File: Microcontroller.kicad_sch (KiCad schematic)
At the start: 87 parts, among them J2 2.54 mm header, J3 Conn_01x14_Pin, J4 HX JN1.27-2x5 WZ H4.9, J5 USB_C_Receptacle_USB2.0_16P, U2 STM32G431K8Tx, U4 USBLC6-2SC6, Y1 20 MHz

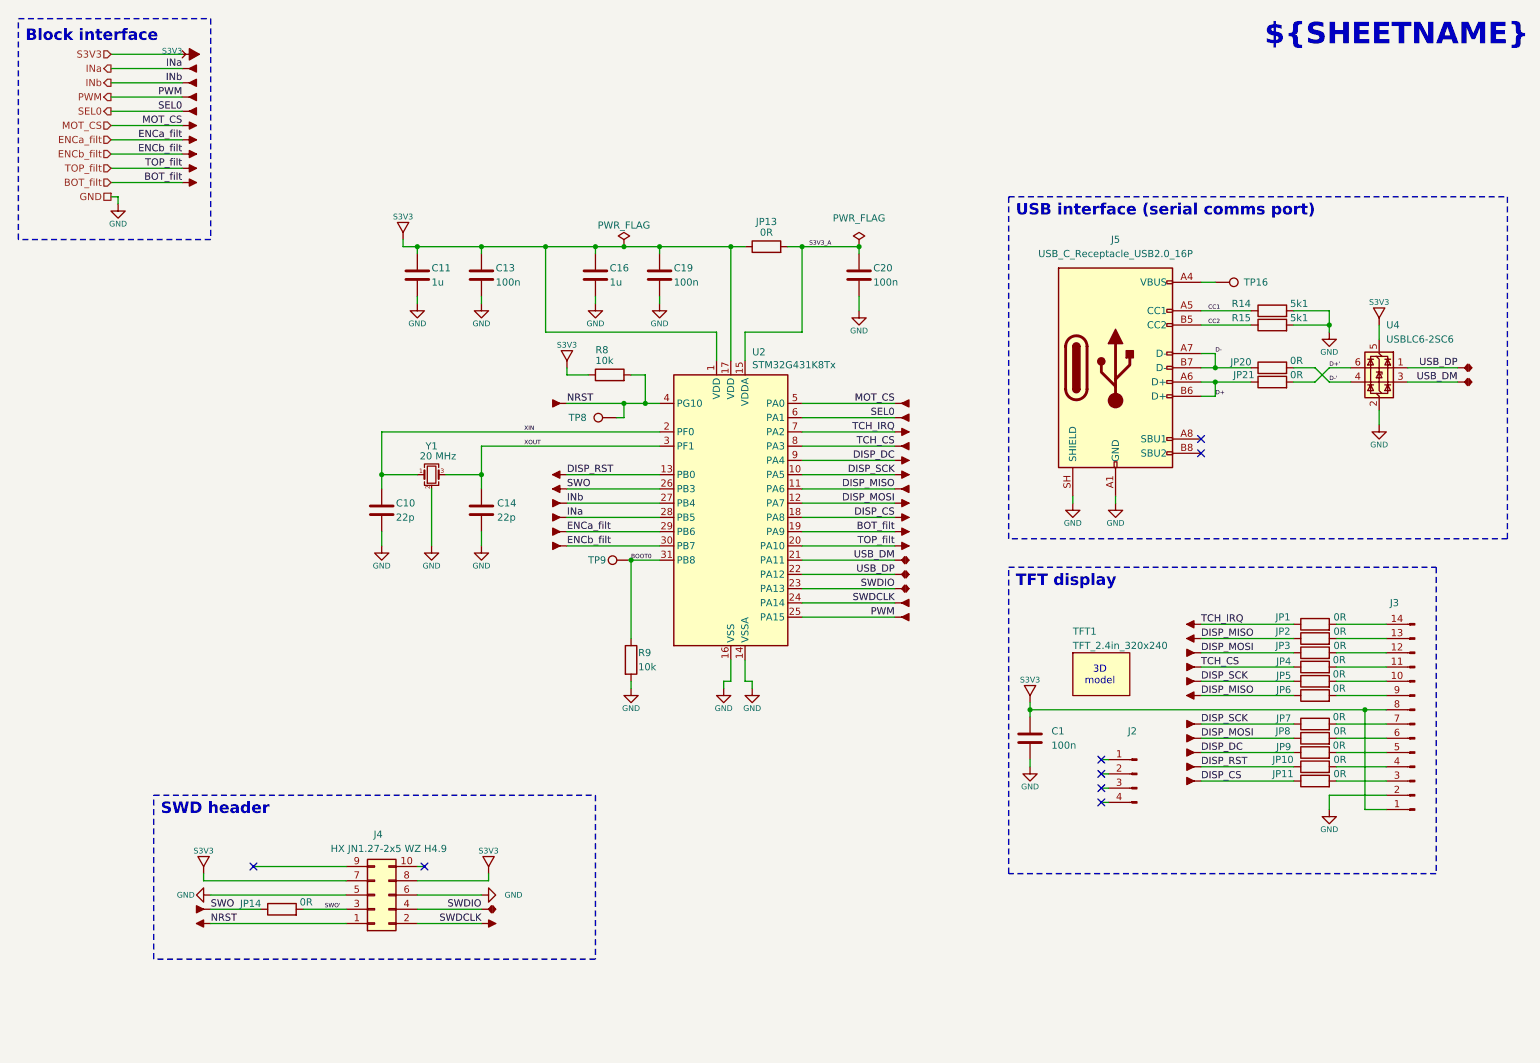
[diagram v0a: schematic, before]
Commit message: sch update
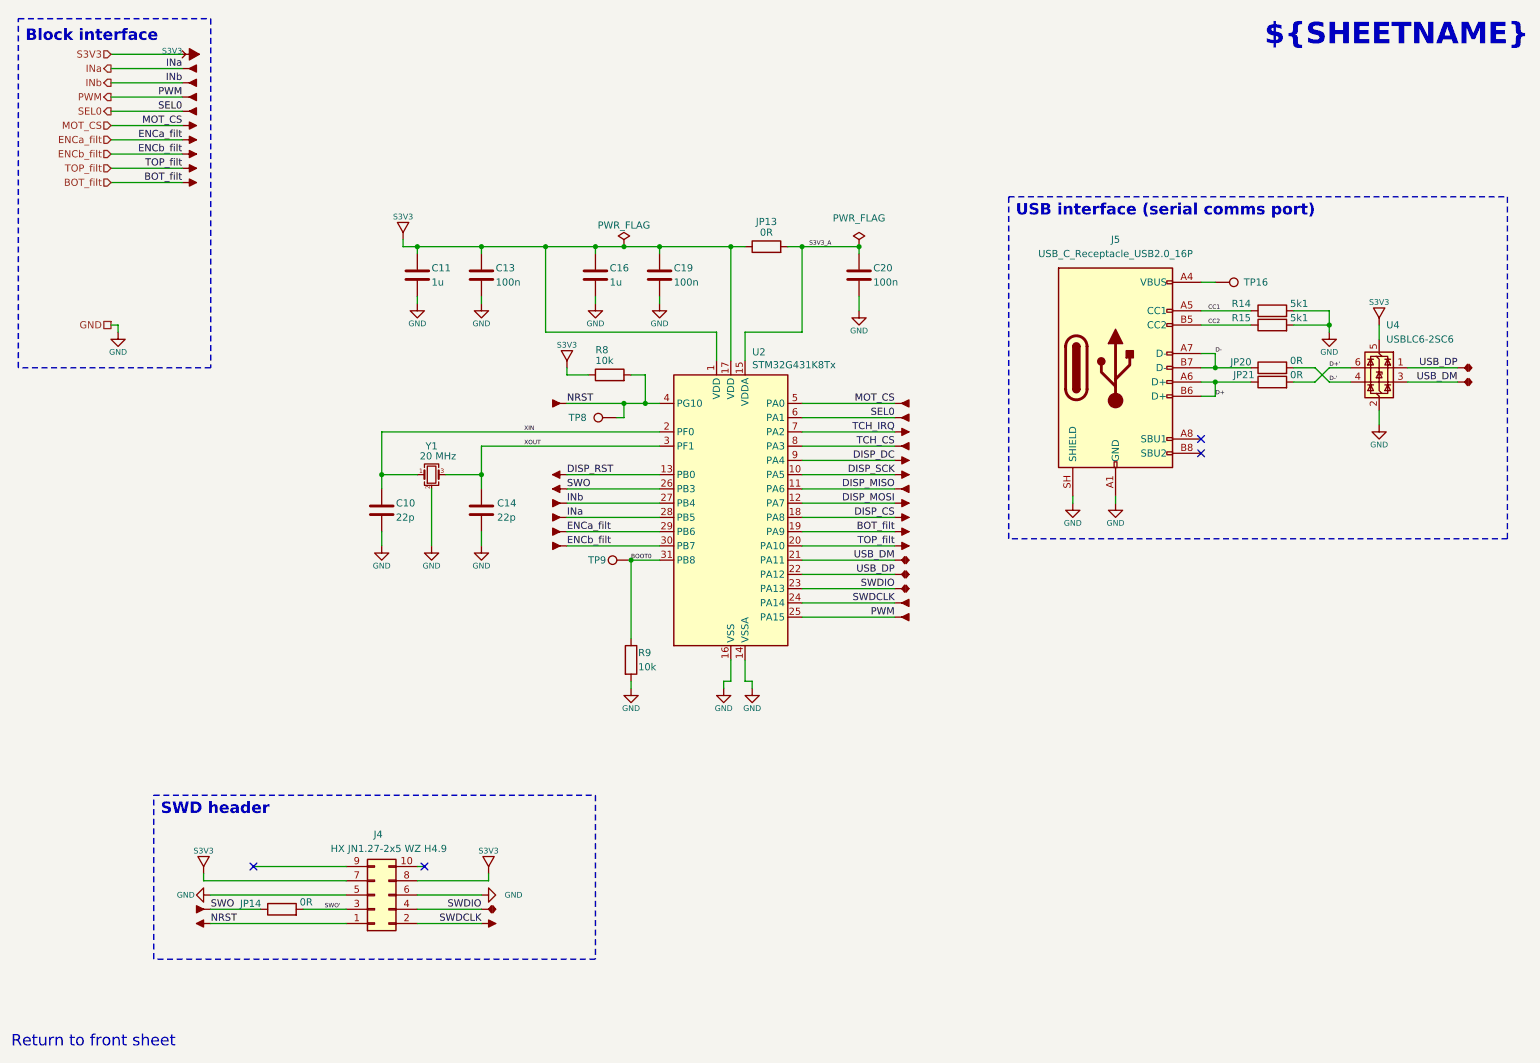
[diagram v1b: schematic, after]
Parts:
- removed C1: 100n, Capacitor_SMD:C_0603_1608Metric_Pad1.08x0.95mm_HandSolder, symbol Device:C
- removed J2: 2.54 mm header, Connector_PinSocket_2.54mm:PinSocket_1x04_P2.54mm_Vertical, symbol Connector:Conn_01x04_Pin
- removed J3: Conn_01x14_Pin, Connector_PinSocket_2.54mm:PinSocket_1x14_P2.54mm_Vertical, symbol Connector:Conn_01x14_Pin
- removed JP1, JP10, JP11, JP2, JP3, JP8: 0R, Personal:Jumper_0603, symbol Device:R
- removed JP4, JP5, JP7: 0R, Resistor_SMD:R_1206_3216Metric_Pad1.30x1.75mm_HandSolder, symbol Device:R
- removed JP6: 0R, Resistor_SMD:R_0603_1608Metric_Pad0.98x0.95mm_HandSolder, symbol Device:R
- removed JP9: 0R, Resistor_THT:R_Axial_DIN0204_L3.6mm_D1.6mm_P5.08mm_Horizontal, symbol Device:R
- removed P1, P2, P6: (no value), symbol personal:Cosmetic_OUT
- removed P10, P11, P3, P4, P5, P7, P8, P9: (no value), symbol personal:Cosmetic_IN
- removed TFT1: TFT_2.4in_320x240, Personal:Display_240x320_ILI9341_2.4in_no_pads, symbol personal:TFT_2.8_IN_320x240
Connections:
- no-connect marks 8 -> 4
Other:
- note added: "Return to front sheet"
- note removed: "3D model"
- note removed: "TFT display"

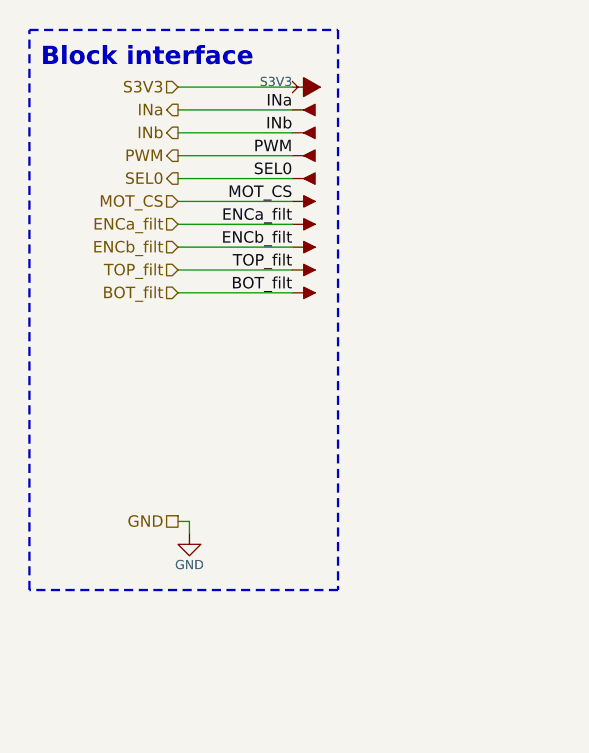
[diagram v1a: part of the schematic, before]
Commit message: sch2
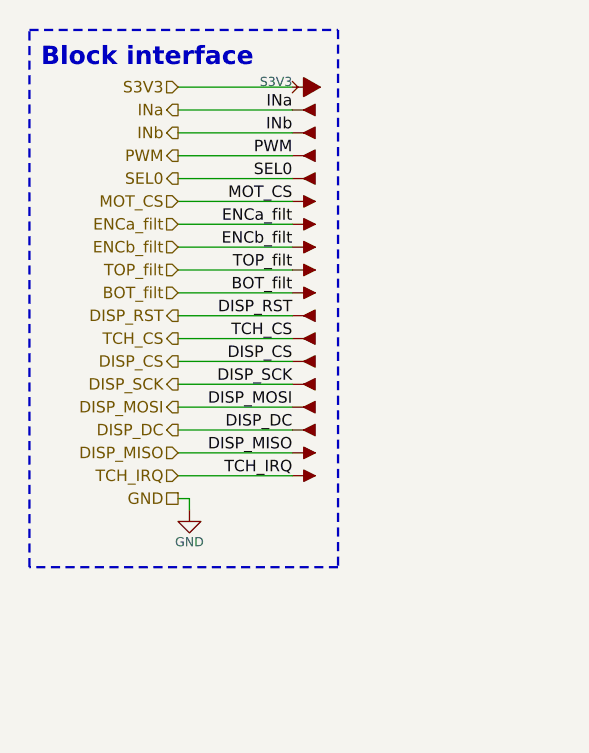
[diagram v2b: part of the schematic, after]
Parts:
- added P100, P101: (no value), symbol personal:Cosmetic_OUT
- added P94, P95, P96, P97, P98, P99: (no value), symbol personal:Cosmetic_IN
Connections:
- net DISP_CS: now also P96.1
- net DISP_DC: now also P99.1
- net DISP_MISO: now also P100.1
- net DISP_MOSI: now also P98.1
- net DISP_RST: now also P94.1
- net DISP_SCK: now also P97.1
- net TCH_CS: now also P95.1
- net TCH_IRQ: now also P101.1

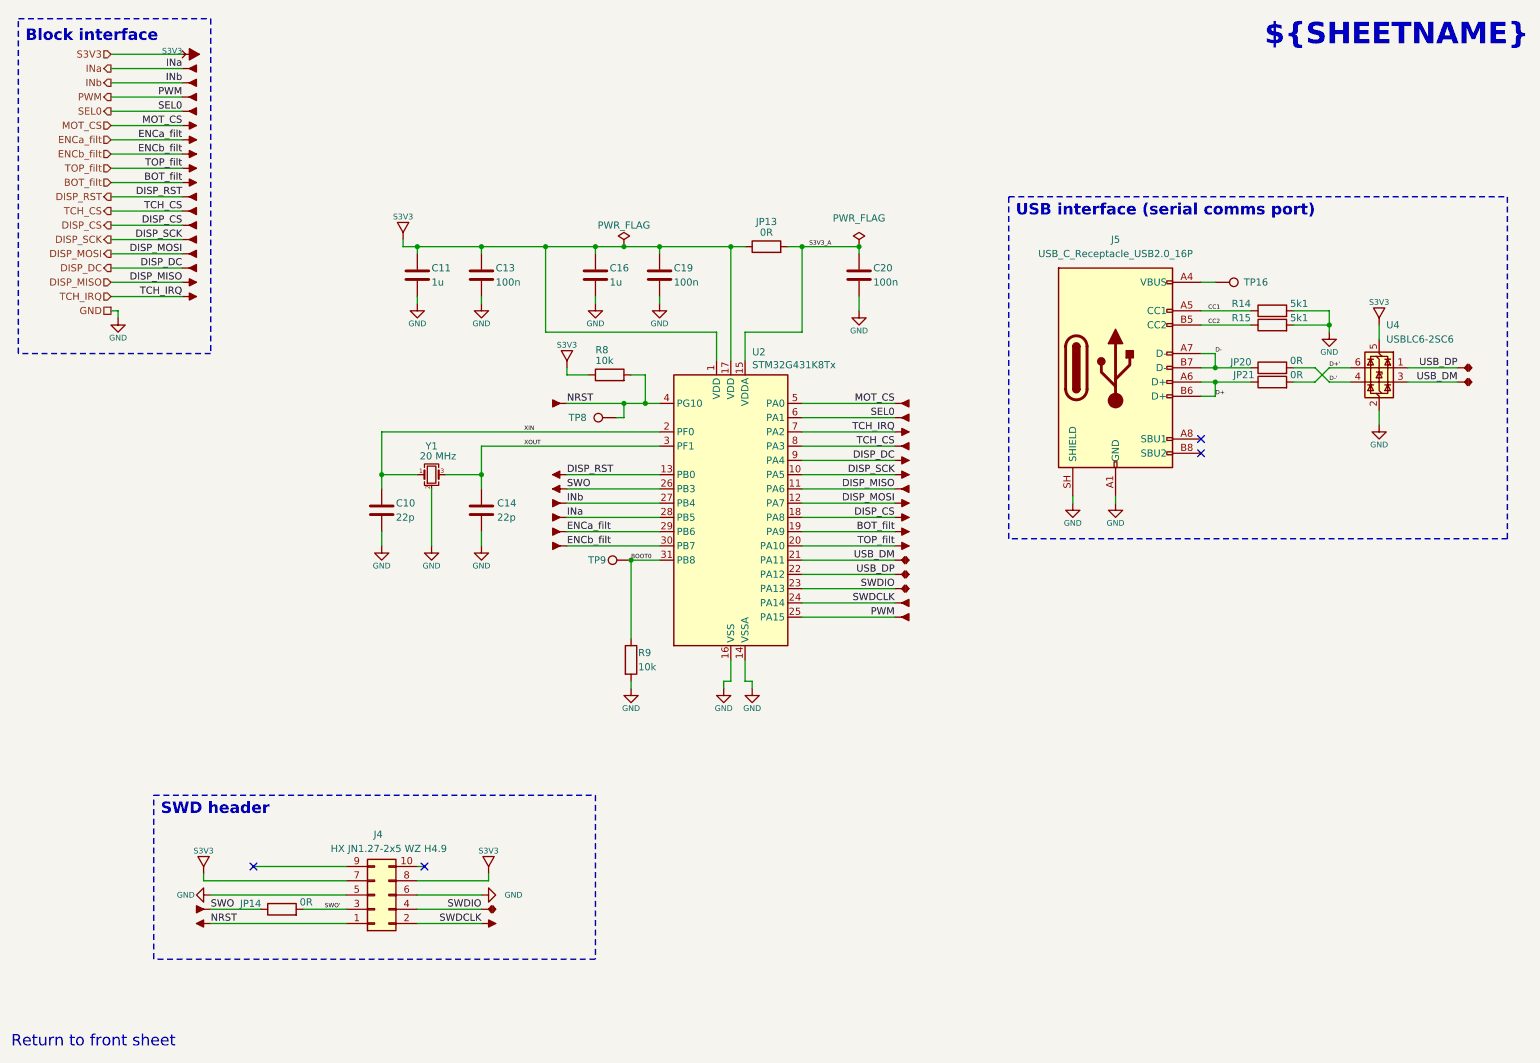
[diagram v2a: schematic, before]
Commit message: reorganised sch and pcb
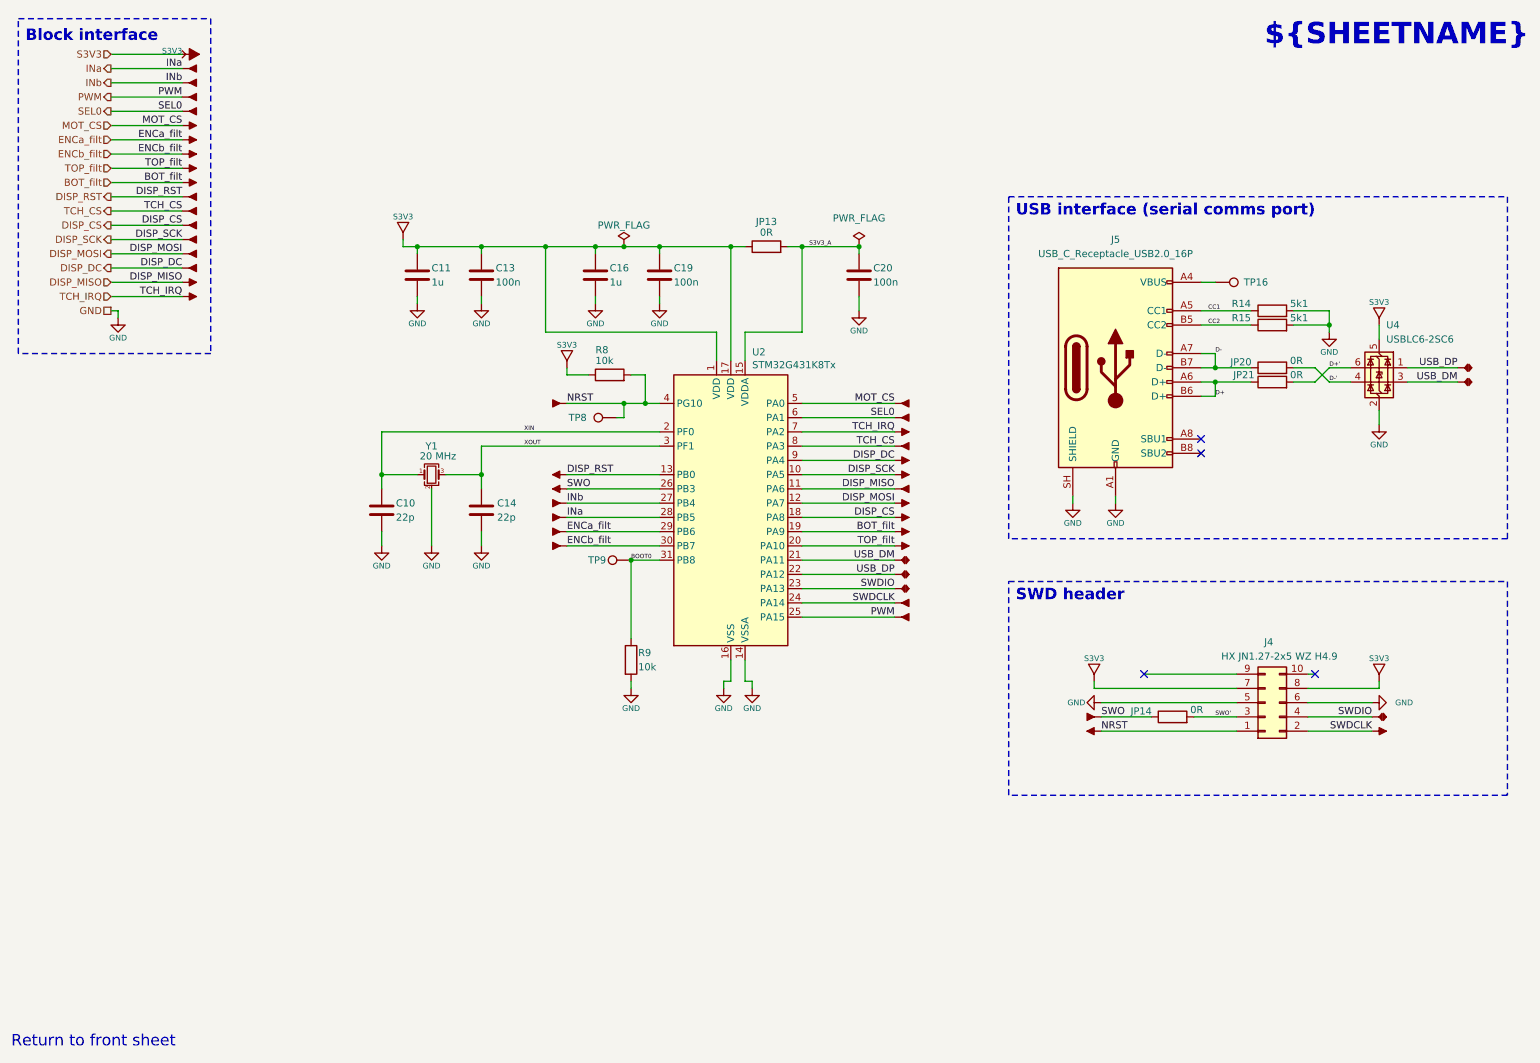
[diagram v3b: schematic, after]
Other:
- moved on the sheet: J4, JP14
